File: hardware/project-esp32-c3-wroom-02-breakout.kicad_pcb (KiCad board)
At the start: 4 copper layers, 25.4 x 24.4 mm, 19 parts, among them J1 SM04B-SRSS-TB(LF)(SN), J2 Conn_01x08_Male, J3 Conn_01x08_Male, Q1 MUN5214DW1T1G, U1 XC6220B331MR, U2 ESP32-C3-WROOM-02-H4

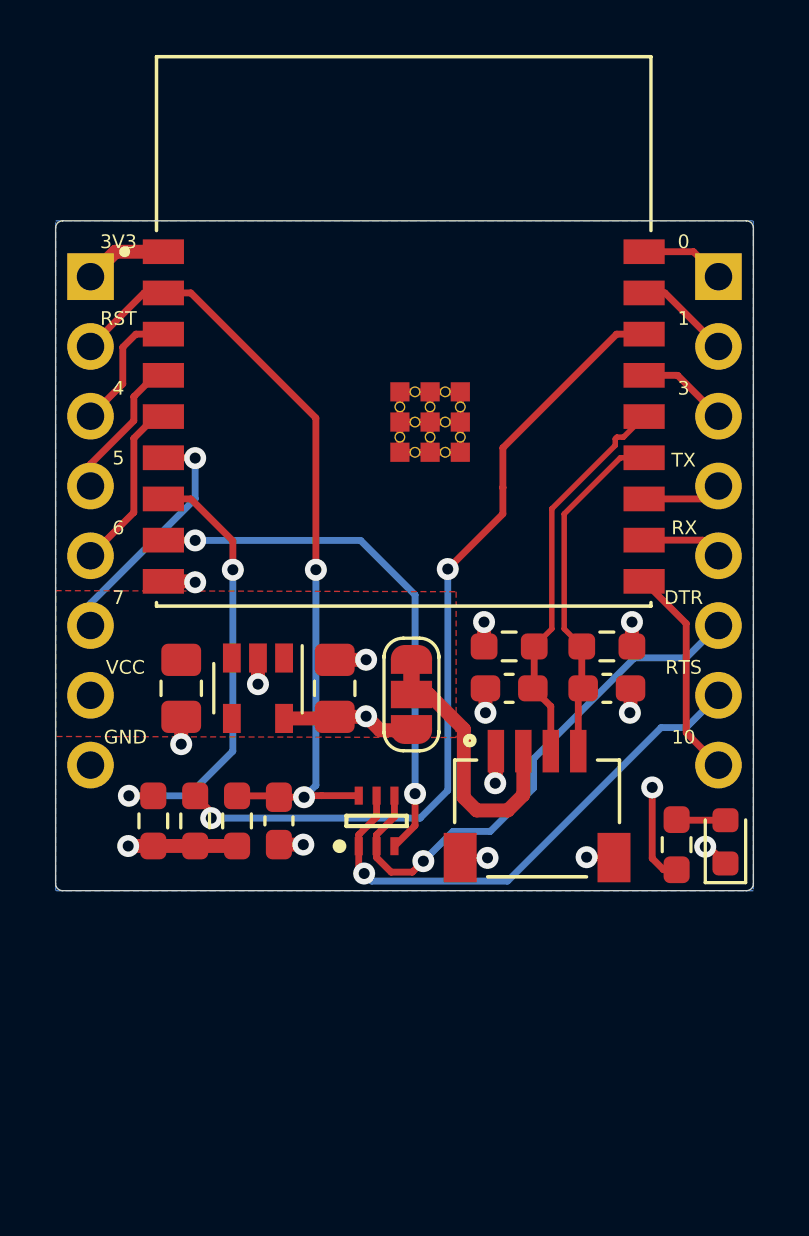
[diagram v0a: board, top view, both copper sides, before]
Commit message: First placement done
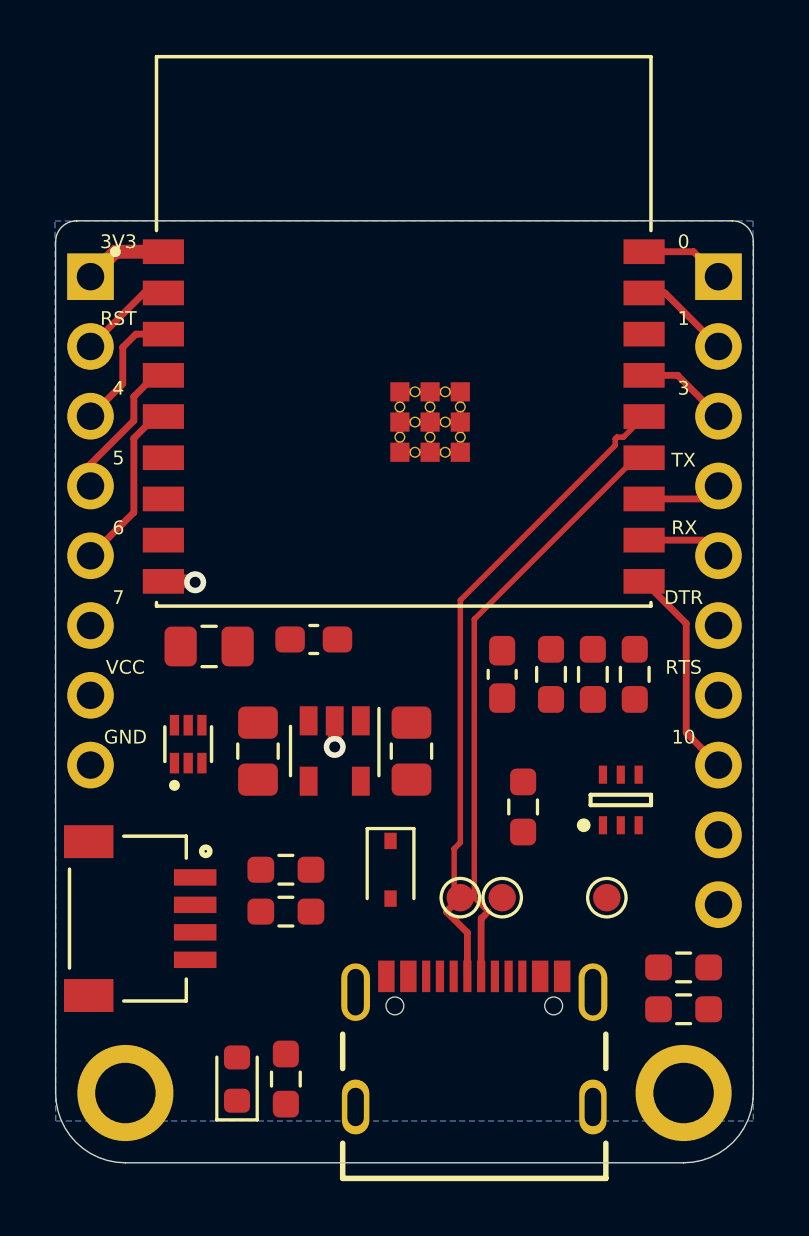
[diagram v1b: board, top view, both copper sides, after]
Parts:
- removed C6: 22pF, Capacitor_SMD:C_0603_1608Metric_Pad1.08x0.95mm_HandSolder
- removed JP1: SolderJumper_3_Bridged12, Jumper:SolderJumper-3_P1.3mm_Bridged12_RoundedPad1.0x1.5mm
- added C3: 0.1uF, Capacitor_SMD:C_0603_1608Metric_Pad1.08x0.95mm_HandSolder, F.Cu at (46.7, 49.0)
- added D2: CUS10S30,H3F‎, Diode_SMD:D_SOD-323, F.Cu at (49.5, 57.4)
- added H1: MountingHole_Pad, MountingHole:MountingHole_2.2mm_M2_ISO7380_Pad, F.Cu at (39.9, 65.5)
- added H2: MountingHole_Pad, MountingHole:MountingHole_2.2mm_M2_ISO7380_Pad, F.Cu at (60.2, 65.5)
- added J4: USB4105-GF-A, USB4105-GF-A:GCT_USB4105-GF-A, F.Cu at (52.6, 66.0)
- added Q2: Q_PMOS_DGS, SSM6J214FE-TE85L-F:SOT50P160X60-6N, F.Cu at (42.2, 52.8)
- added R7: 100k, Resistor_SMD:R_0603_1608Metric_Pad0.98x0.95mm_HandSolder, F.Cu at (54.4, 55.1)
- added R8: 5.1k, Resistor_SMD:R_0603_1608Metric_Pad0.98x0.95mm_HandSolder, F.Cu at (60.2, 62.5)
- added R9: 5.1k, Resistor_SMD:R_0603_1608Metric_Pad0.98x0.95mm_HandSolder, F.Cu at (60.2, 61.0)
- added TP1: TestPoint, TestPoint:TestPoint_Pad_D1.0mm, F.Cu at (52.1, 58.4)
- added TP2: TestPoint, TestPoint:TestPoint_Pad_D1.0mm, F.Cu at (53.6, 58.4)
- added TP3: TestPoint, TestPoint:TestPoint_Pad_D1.0mm, F.Cu at (57.4, 58.4)
- C1, C4: value 10uF -> 22uF
- C5: value 22pF -> 22uF; footprint Capacitor_SMD:C_0603_1608Metric_Pad1.08x0.95mm_HandSolder -> Capacitor_SMD:C_0805_2012Metric_Pad1.18x1.45mm_HandSolder
- J3: value Conn_01x08_Male -> Conn_01x10_Male; footprint Connector_PinHeader_2.54mm:PinHeader_1x08_P2.54mm_Vertical -> Connector_PinHeader_2.54mm:PinHeader_1x10_P2.54mm_Vertical
- R4, R5: value 4k7 -> 5.1k
- R6: value 10k -> 5.1k
- moved D1 19.8 mm to (43.9, 65.0)
- moved R2 16.9 mm to (58.4, 50.3)
- moved R3 16.9 mm to (56.9, 50.3)
- moved R6 16.6 mm to (45.7, 65.0)
- moved R4 15.2 mm to (45.7, 58.9)
- moved J1 13.9 mm to (42.4, 59.2), turned to 270 degrees
- moved R1 12.6 mm to (55.4, 50.3)
- moved R5 11.5 mm to (45.7, 57.4), turned to 180 degrees
- moved C5 11.0 mm to (42.9, 49.3)
- moved C2 9.72 mm to (53.6, 50.3)
- moved Q1 8.92 mm to (57.9, 54.9)
- moved C1 3.61 mm to (44.7, 53.1)
- moved C4 3.61 mm to (50.3, 53.1)
- moved U1 3.61 mm to (47.5, 53.1)
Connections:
- C1 pad 1: VCC -> Net-(C1-Pad1)
- C5 pad 1: /USB_D+ -> +3V3
- J1 pad 2: Net-(J1-Pad2) -> +3V3
- J1 pad 3: /USB_D+ -> /SDA
- J1 pad 4: /USB_D- -> /SCL
- J2 pad 5: /GPIO6 -> /SDA
- J2 pad 6: /GPIO7 -> /SCL
- J2 pad 7: VCC -> +BATT
- R4 pad 2: /USB_D- -> /SCL
- R5 pad 2: /USB_D+ -> /SDA
- U1 pad 1: VCC -> Net-(C1-Pad1)
- U1 pad 3: VCC -> Net-(C1-Pad1)
- U2 pad 5: /GPIO6 -> /SDA
- U2 pad 6: /GPIO7 -> /SCL
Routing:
- net /GPIO2: track 30.3 -> 0.00 mm, vias 2 -> 0
- net /RESET: track 29.4 -> 3.46 mm, vias 2 -> 0
- net /DTR: track 19.7 -> 0.00 mm, vias 1 -> 0
- net /GPIO9: track 19.4 -> 0.00 mm, vias 2 -> 0
- net /RTS: track 19.0 -> 0.00 mm, vias 1 -> 0
- net /GPIO8: track 16.2 -> 0.00 mm, vias 2 -> 0
- net +3V3: track 17.3 -> 3.03 mm, vias 5 -> 0
- net /USB_D+: track 14.3 -> 23.8 mm
- net /USB_D-: track 12.8 -> 21.9 mm
- net Net-(J1-Pad2): track 9.11 -> 0.00 mm
- net GND: track 24.3 -> 15.3 mm, vias 11 -> 2
- net /GPIO7: track 8.84 -> 0.00 mm, vias 1 -> 0
- net /SDA: track 0.00 -> 6.33 mm
- net /GPIO6: track 6.33 -> 0.00 mm
- net Net-(D1-Pad2): track 1.79 -> 0.00 mm
- removed copper zone on F.Cu, net VCC
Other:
- board size 25.4 x 24.4 mm -> 25.4 x 34.3 mm
